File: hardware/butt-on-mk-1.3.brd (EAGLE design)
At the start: 22.9 x 17.8 mm, 13 parts, among them U1_ ROTARY_ENCODER_SWITCH, U2 Tiny85

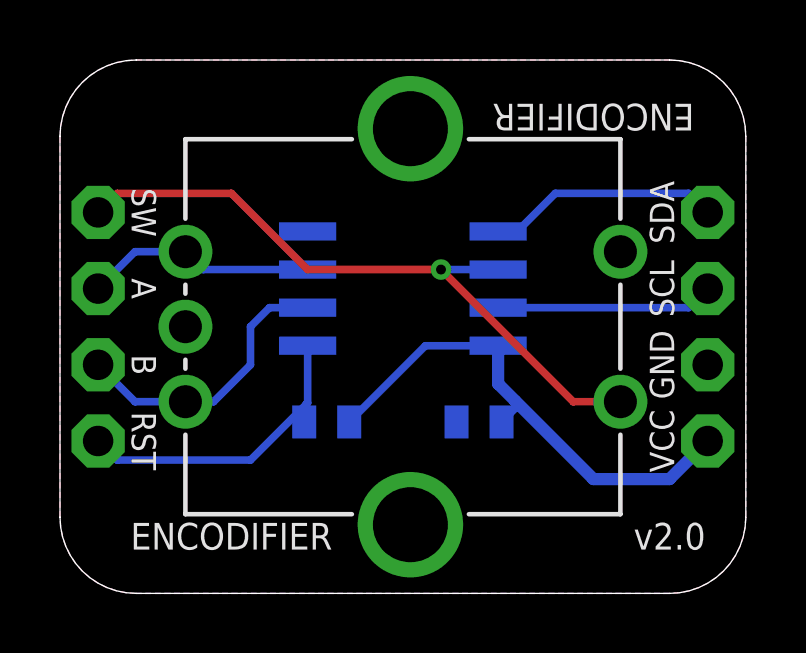
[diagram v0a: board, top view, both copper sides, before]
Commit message: have some boards, dawg
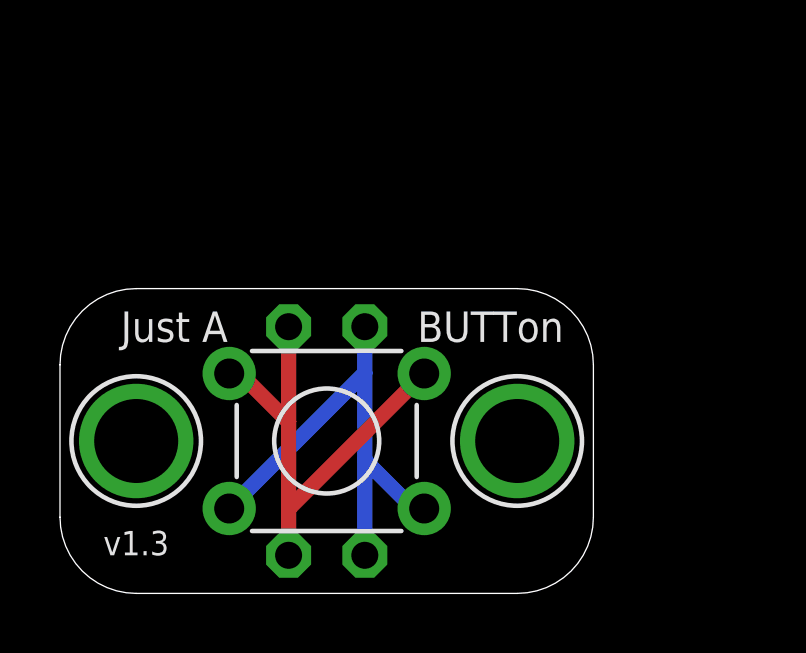
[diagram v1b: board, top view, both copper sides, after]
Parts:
- removed A, B, GND, RST, SCL, SDA, SW, VCC: M01PTH-1MM, a_parts:1X01-1MM-NS
- removed C1: 100n, a_parts:C0603-TIGHTER
- removed R1: 10k, a_parts:R0603-TIGHTER
- removed U1_: ROTARY_ENCODER_SWITCH, a_parts:ROTARY_ENCODER_SWITCH
- removed U2: Tiny85, a_parts:SO08-EIAJ
- added JP1, JP2, JP3, JP4: M01PTH-0.9MM-NS, a_parts:1X01-0.9MM-NS
- added S1: SPST-NO-TACT6MM-PTH-SMALL-PADS, a_parts:DTS-6-SMALL-PADS
- FRAME1: device A_butts:DUMMY -> a_parts:DUMMY
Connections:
- removed net A: A.1, U1_.A, U2.3
- removed net B: B.1, U1_.B, U2.2
- removed net GND: C1.2, GND.1, U1_.C, U1_.SW2, U2.4
- removed net MOSI/SDA: SDA.1, U2.5
- removed net RST: R1.1, RST.1, U2.1
- removed net SCK/SCL: SCL.1, U2.7
- removed net SW: SW.1, U1_.SW1, U2.6
- removed net VCC: C1.1, R1.2, U2.8, VCC.1
- new net N$1: JP1.1, JP3.1, S1.1, S1.2
- new net N$2: JP2.1, JP4.1, S1.3, S1.4
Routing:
- net SW: track 22.5 -> 0.00 mm, vias 1 -> 0
- net VCC: track 17.0 -> 0.00 mm
- net N$1: track 0.00 -> 16.7 mm
- net N$2: track 0.00 -> 16.7 mm
- net RST: track 10.5 -> 0.00 mm
- net B: track 9.54 -> 0.00 mm
- net MOSI/SDA: track 7.77 -> 0.00 mm
- net A: track 7.74 -> 0.00 mm
- net SCK/SCL: track 7.25 -> 0.00 mm
- removed copper zone on layer 1, net GND
- removed copper zone on layer 16, net GND
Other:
- board size 22.9 x 17.8 mm -> 17.8 x 10.2 mm
- board text added: "BUTTon"
- board text added: "Just A"
- board text added: "Now with"
- board text added: "screw holes!"
- board text removed: "C"
- board text removed: "COM"
- board text removed: "ENCODIFIER"
- board text removed: "SW"
